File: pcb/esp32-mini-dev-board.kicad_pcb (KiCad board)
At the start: 4 copper layers, 31 x 38.3 mm, 32 parts, among them J1 USB_C_Receptacle_USB2.0_16P, J2 Conn_01x08_Pin, J3 Conn_01x08_Pin, SW1 SW_Push, SW2 SW_Push, U1 USBLC6-2SC6, U2 AP2112K-3.3, U3 ESP32-C3-WROOM-02, Y1 Crystal

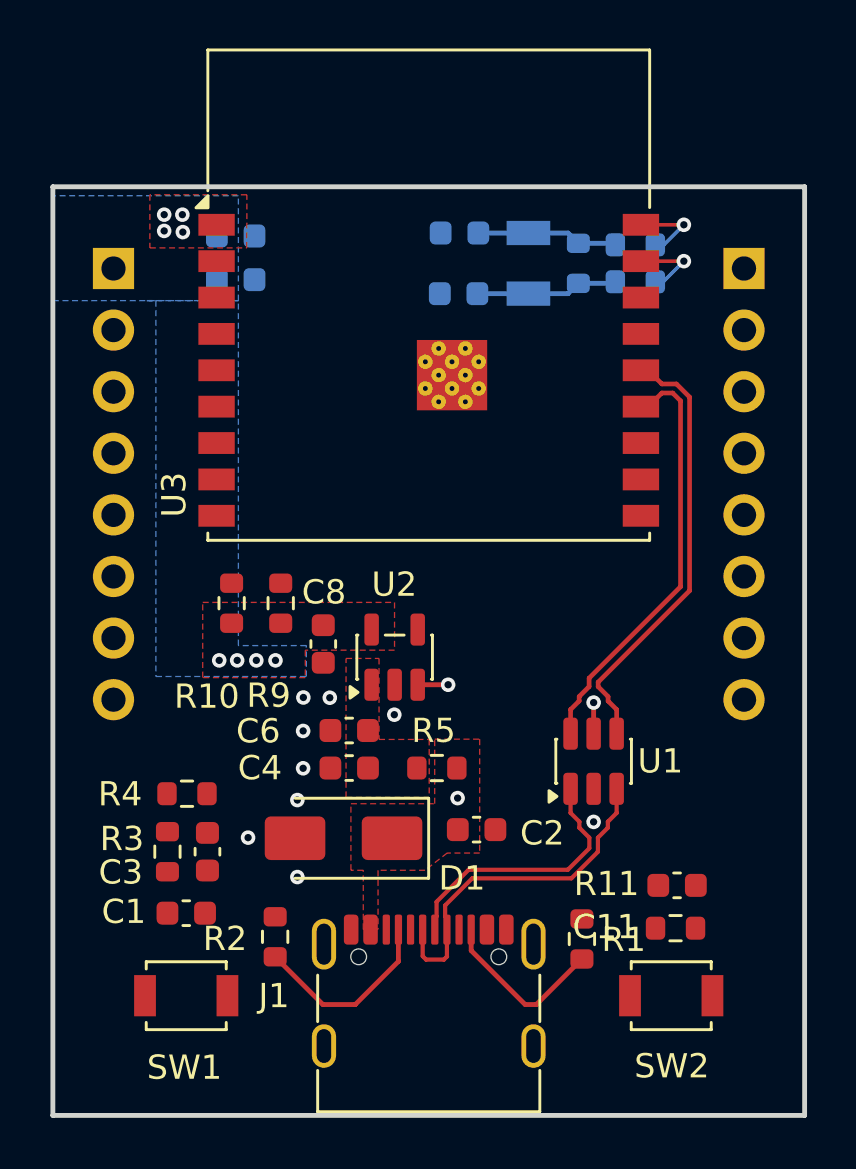
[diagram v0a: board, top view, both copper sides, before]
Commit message: feat(lay): finish routing and copper pouring
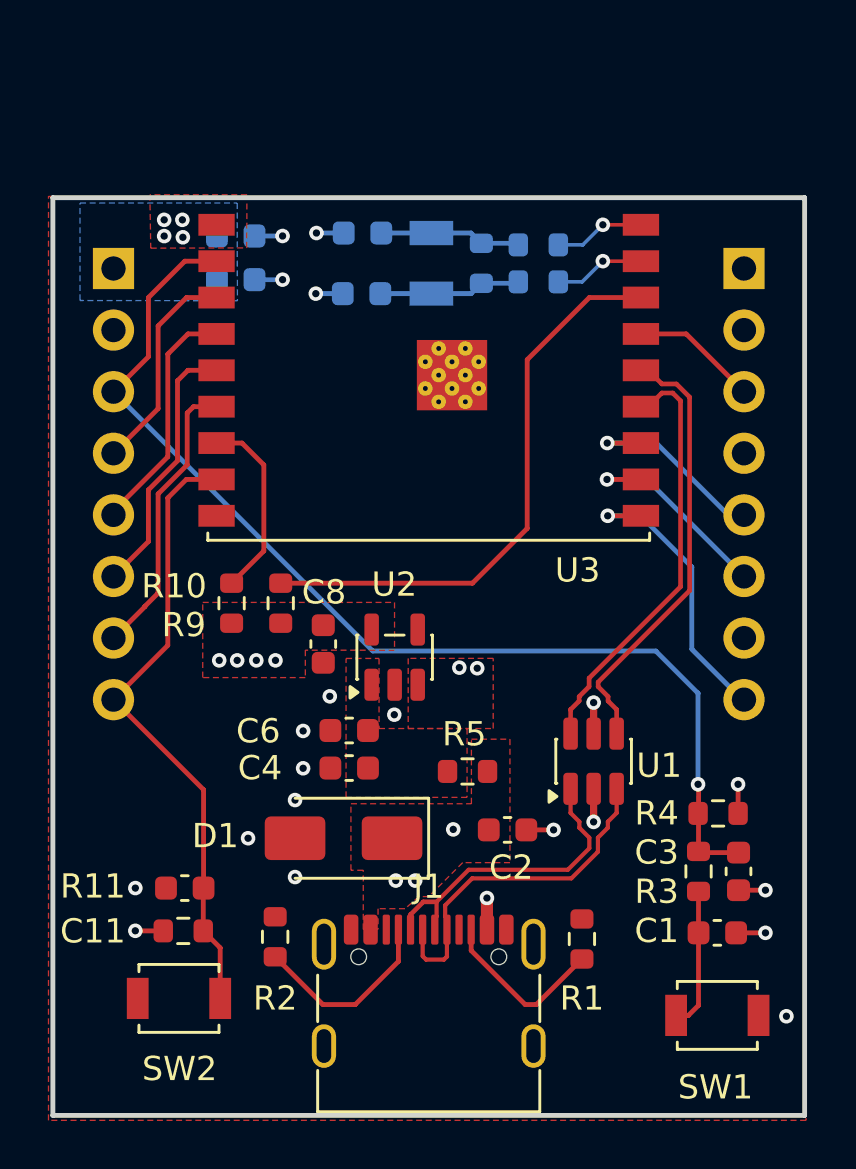
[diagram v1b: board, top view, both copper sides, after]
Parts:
- J1: footprint Connector_USB:USB_C_Receptacle_G-Switch_GT-USB-7010ASV -> CONNECTORS:USB_C_Receptacle_G-Switch_GT-USB-7010ASV
- moved C1 21.9 mm to (174.9, 127.4)
- moved C3 21.9 mm to (175.8, 124.9)
- moved R3 21.9 mm to (174.1, 124.9)
- moved R4 21.9 mm to (174.9, 122.5)
- moved SW1 21.9 mm to (174.9, 130.8)
- moved R11 20.3 mm to (152.9, 127.3)
- moved SW2 20.3 mm to (152.7, 130.1)
- moved C11 20.3 mm to (152.9, 125.6)
- moved C5 4.00 mm to (160.3, 98.5)
- moved C7 4.00 mm to (160.2, 101.0)
- moved R6 4.00 mm to (167.5, 99.0)
- moved R7 4.00 mm to (165.2, 99.8)
- moved R8 4.00 mm to (167.5, 100.5)
- moved Y1 4.00 mm to (163.1, 99.8)
- moved C2 1.28 mm to (166.2, 123.2)
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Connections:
- C3 pad 1: /CIRCUIT DESIGN/EN_RST -> /CIRCUIT DESIGN/EN
- R3 pad 2: /CIRCUIT DESIGN/EN_RST -> /CIRCUIT DESIGN/EN
- R4 pad 2: /CIRCUIT DESIGN/EN_RST -> /CIRCUIT DESIGN/EN
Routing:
- net /CIRCUIT DESIGN/EN: track 0.00 -> 45.4 mm, vias 0 -> 1
- net +3V3: track 0.00 -> 37.0 mm, vias 8 -> 10
- net /CIRCUIT DESIGN/BOOT: track 0.00 -> 25.7 mm
- net Net-(U3-IO2): track 0.00 -> 23.8 mm
- net /CIRCUIT DESIGN/IO10: track 0.00 -> 12.1 mm, vias 0 -> 1
- net /CIRCUIT DESIGN/IO7: track 0.00 -> 11.9 mm
- net /CIRCUIT DESIGN/IO6: track 0.00 -> 11.0 mm
- net /CIRCUIT DESIGN/IO5: track 0.00 -> 9.91 mm
- net GND: track 0.00 -> 9.36 mm, vias 9 -> 17
- net /CIRCUIT DESIGN/IO4: track 0.00 -> 8.91 mm
- net /CIRCUIT DESIGN/RXD: track 0.00 -> 8.71 mm, vias 0 -> 1
- net /CIRCUIT DESIGN/TXD: track 0.00 -> 8.26 mm, vias 0 -> 1
- net Net-(U3-IO8): track 0.00 -> 7.75 mm
- net Net-(C1-Pad1): track 0.00 -> 5.79 mm
- net /CIRCUIT DESIGN/IO3: track 0.00 -> 5.24 mm
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- added copper zone on In2.Cu, net +3V3
- added copper zone on In2.Cu, net +5V
- added copper zone on In2.Cu, net /CIRCUIT DESIGN/VBUS
- added copper zone on F.Cu, net GND
- added copper zone on In1.Cu, net GND
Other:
- board size 31 x 38.3 mm -> 31 x 37.8 mm
